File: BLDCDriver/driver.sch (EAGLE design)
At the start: 54 parts, among them Q1 NJM7800S, U1 QFN50P400X400X100-25NDRV8300D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, U2 AS5048A-HTSP-500, U4 SOP80P620X125-8N

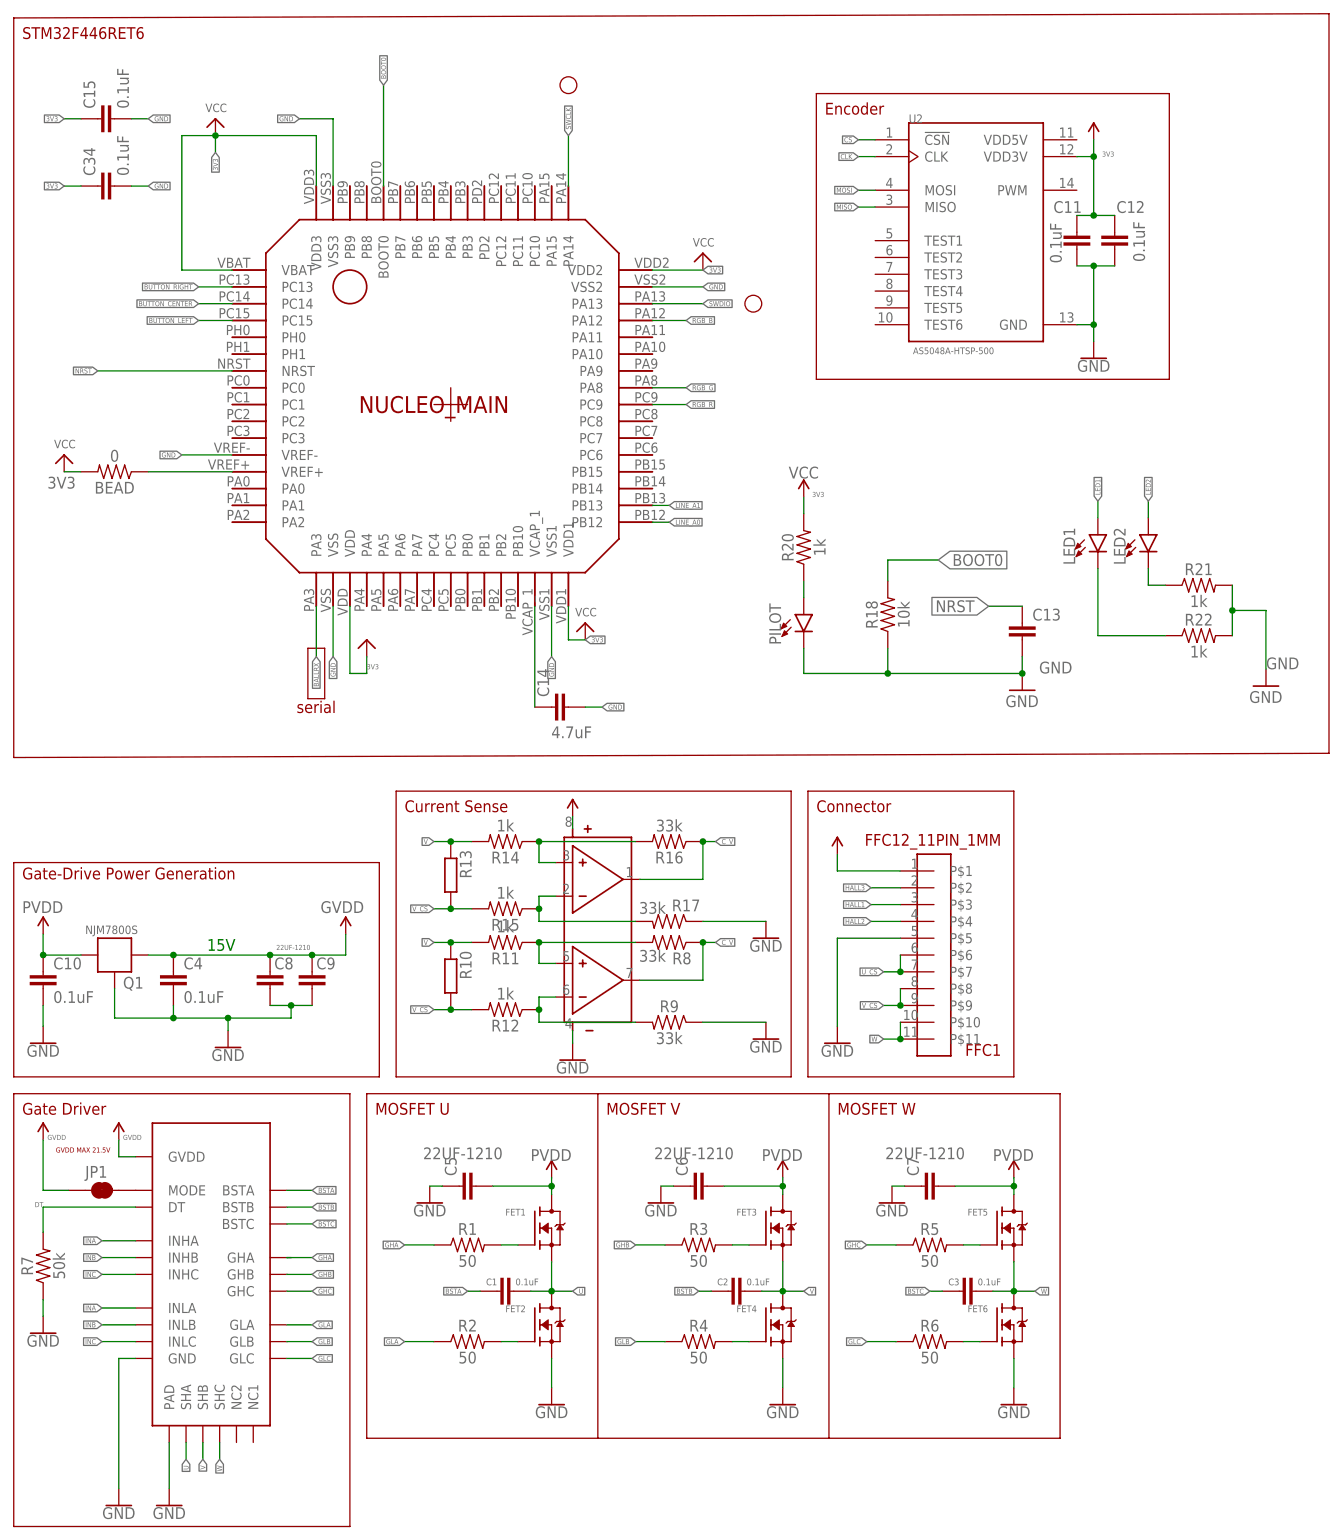
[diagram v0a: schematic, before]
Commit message: somefix
# ==== Emojis ====
# ✨ :sparkles: Add new feature
# ✅  :white_check_mark: Update existing feature (not bug)
# ⚠️  :warning: Fix bug/error
# 🔥  :fire: Remove files or features
# ✏️ :pencil2: Fix typos
# 📝  :memo: Update documentation
# ♻️  :recycle: Dependencies update
# 🐧  :penguin: Improved the Linux
# 🍎  :apple: Improved the macOS
# 🔖 :bookmark: Add new library
# 🎉  :tada: Initial commit

# ==== Format ====
# :emoji: Subject
#
# Commit body...

# ==== Messages ====
# 新規(ファイル)機能追加: Add
# 機能修正、既存機能追加（バグではない): Update
# リファクタリング: Clean
# ファイル名変更:
# 削除など: Remove
# バグ修正: Fix
# バージョンアップ: Upgrade
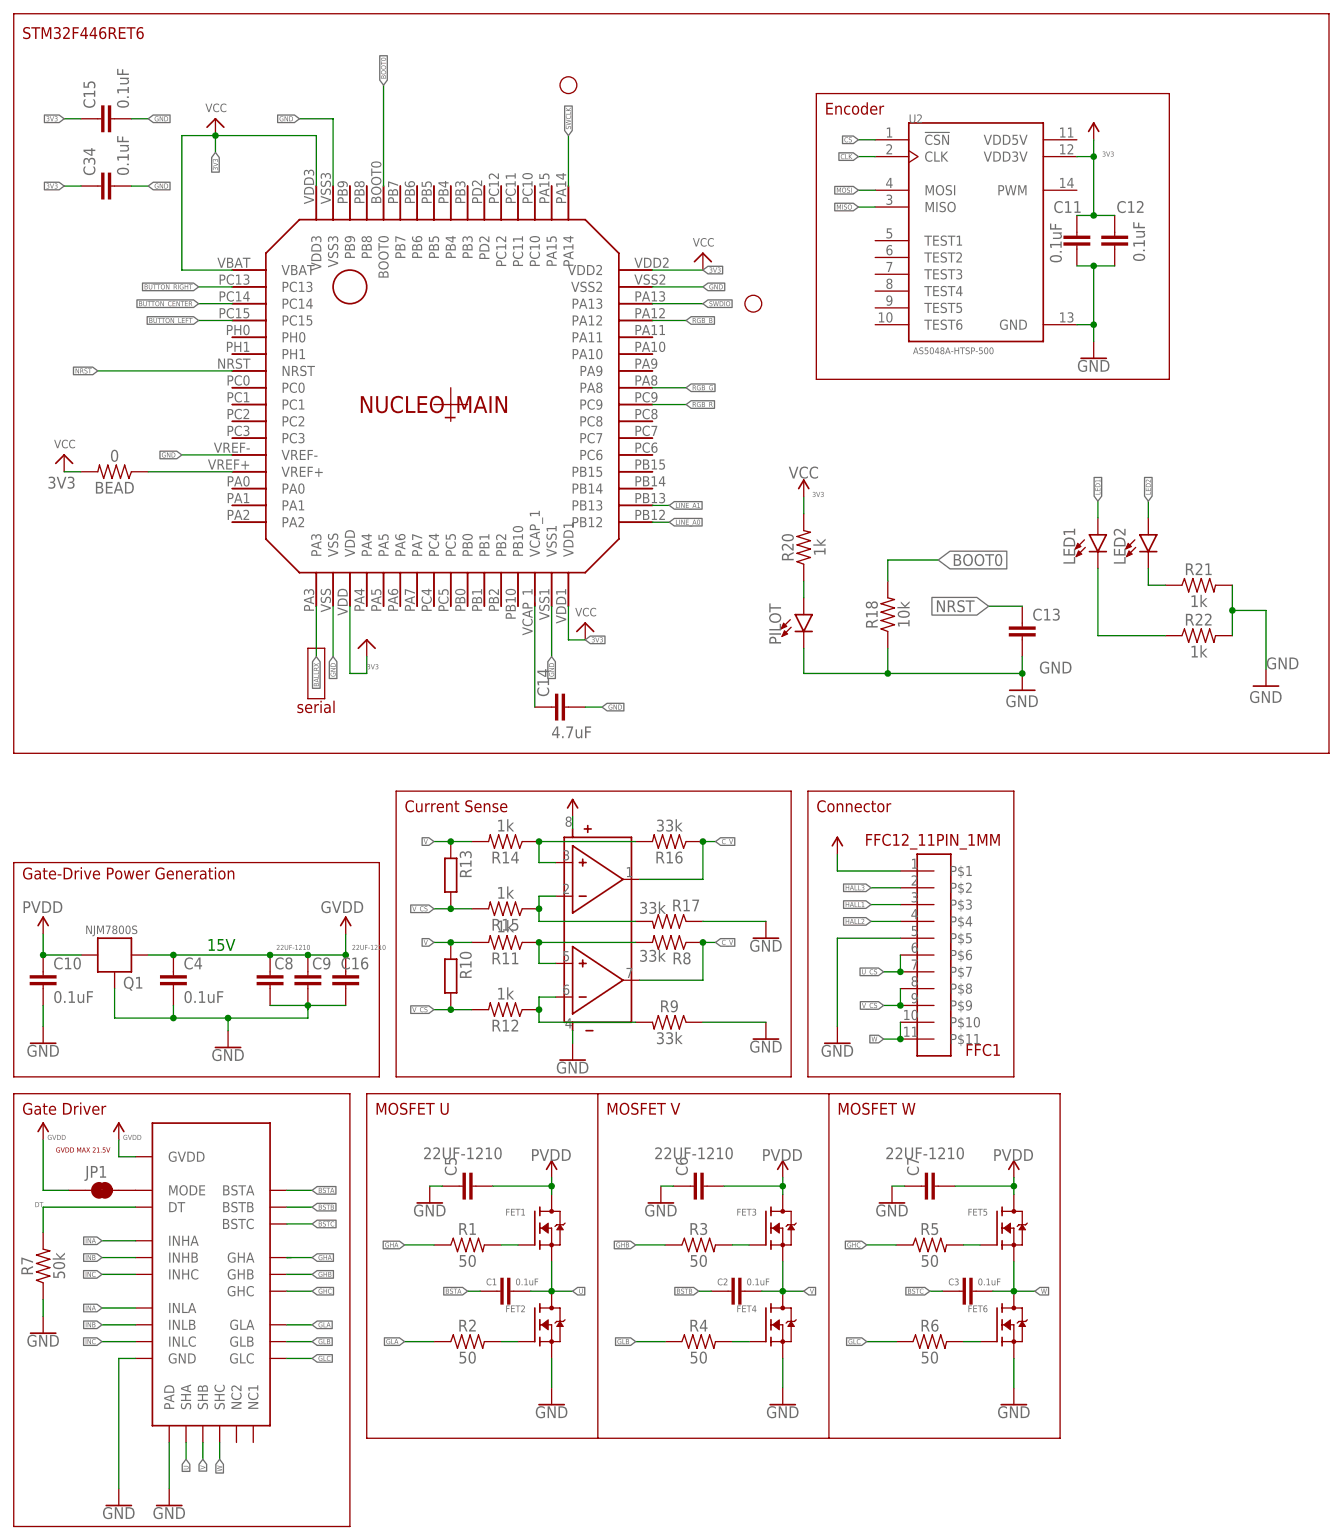
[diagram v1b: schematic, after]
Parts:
- added C16: 22UF-1210, SparkFun-Capacitors:22UF-1210-16V-20%
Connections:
- net GND: now also C16.1
- net GVDD: now also C16.2
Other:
- moved on the sheet: C9
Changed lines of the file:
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@@
 <part name="P+6" library="audio amplifier example" library_urn="urn:adsk.eagle:library:970892" deviceset="VCC" device=""/>
 <part name="GND18" library="supply" deviceset="GND" device=""/>
+<part name="C16" library="SparkFun-Capacitors" deviceset="22UF" device="-1210-16V-20%" value="22UF-1210"/>
 </parts>
 <sheets>
@@
 <circle x="83.82" y="217.805" radius="1.27" width="0.1524" layer="94"/>
 <circle x="111.76" y="184.785" radius="1.27" width="0.1524" layer="94"/>
-<wire x1="0" y1="227.965" x2="0" y2="116.205" width="0.1524" layer="94"/>
-<wire x1="0" y1="116.205" x2="198.755" y2="116.84" width="0.1524" layer="94"/>
+<wire x1="0" y1="228.6" x2="0" y2="116.84" width="0.1524" layer="94"/>
+<wire x1="0" y1="116.84" x2="198.755" y2="116.84" width="0.1524" layer="94"/>
 <wire x1="198.755" y1="116.84" x2="198.755" y2="228.6" width="0.1524" layer="94"/>
-<wire x1="198.755" y1="228.6" x2="0" y2="227.965" width="0.1524" layer="94"/>
+<wire x1="198.755" y1="228.6" x2="0" y2="228.6" width="0.1524" layer="94"/>
 <text x="1.27" y="224.79" size="1.778" layer="94">STM32F446RET6</text>
 </plain>
@@
 <attribute name="VALUE" x="44.831" y="87.884" size="0.762" layer="96" font="vector" rot="R180"/>
 </instance>
-<instance part="C9" gate="G$1" x="45.085" y="83.82" smashed="yes" rot="R180">
-<attribute name="NAME" x="48.641" y="85.979" size="1.778" layer="95" font="vector" rot="R180"/>
+<instance part="C9" gate="G$1" x="44.45" y="83.82" smashed="yes" rot="R180">
+<attribute name="NAME" x="48.006" y="85.979" size="1.778" layer="95" font="vector" rot="R180"/>
 </instance>
 <instance part="GND6" gate="1" x="32.385" y="72.39" smashed="yes">
@@
 <instance part="GND18" gate="1" x="189.23" y="127" smashed="yes">
 <attribute name="VALUE" x="186.69" y="124.46" size="1.778" layer="96"/>
+</instance>
+<instance part="C16" gate="G$1" x="50.165" y="83.82" smashed="yes" rot="R180">
+<attribute name="NAME" x="53.721" y="85.979" size="1.778" layer="95" font="vector" rot="R180"/>
+<attribute name="VALUE" x="56.261" y="87.884" size="0.762" layer="96" font="vector" rot="R180"/>
 </instance>
 </instances>
@@
 <wire x1="15.24" y1="81.28" x2="15.24" y2="76.835" width="0.1524" layer="91"/>
 <pinref part="C4" gate="G$1" pin="2"/>
-<pinref part="C8" gate="G$1" pin="1"/>
-<pinref part="C9" gate="G$1" pin="1"/>
-<wire x1="38.735" y1="78.74" x2="41.91" y2="78.74" width="0.1524" layer="91"/>
-<wire x1="41.91" y1="78.74" x2="45.085" y2="78.74" width="0.1524" layer="91"/>
-<wire x1="41.91" y1="78.74" x2="41.91" y2="76.835" width="0.1524" layer="91"/>
-<junction x="41.91" y="78.74"/>
 <wire x1="24.13" y1="76.835" x2="24.13" y2="78.74" width="0.1524" layer="91"/>
 <wire x1="24.13" y1="76.835" x2="15.24" y2="76.835" width="0.1524" layer="91"/>
@@
 <pinref part="GND6" gate="1" pin="GND"/>
 <wire x1="24.13" y1="76.835" x2="32.385" y2="76.835" width="0.1524" layer="91"/>
-<wire x1="32.385" y1="76.835" x2="41.91" y2="76.835" width="0.1524" layer="91"/>
+<wire x1="32.385" y1="76.835" x2="44.45" y2="76.835" width="0.1524" layer="91"/>
 <wire x1="32.385" y1="74.93" x2="32.385" y2="76.835" width="0.1524" layer="91"/>
 <junction x="32.385" y="76.835"/>
+<pinref part="C9" gate="G$1" pin="1"/>
+<pinref part="C16" gate="G$1" pin="1"/>
+<wire x1="50.165" y1="78.74" x2="44.45" y2="78.74" width="0.1524" layer="91"/>
+<junction x="44.45" y="78.74"/>
+<pinref part="C8" gate="G$1" pin="1"/>
+<wire x1="38.735" y1="78.74" x2="44.45" y2="78.74" width="0.1524" layer="91"/>
+<wire x1="44.45" y1="78.105" x2="44.45" y2="78.74" width="0.1524" layer="91"/>
+<wire x1="44.45" y1="78.74" x2="44.45" y2="76.835" width="0.1524" layer="91"/>
 </segment>
 <segment>
@@
 <pinref part="C8" gate="G$1" pin="2"/>
 <junction x="38.735" y="86.36"/>
-<wire x1="38.735" y1="86.36" x2="45.085" y2="86.36" width="0.1524" layer="91"/>
+<wire x1="38.735" y1="86.36" x2="44.45" y2="86.36" width="0.1524" layer="91"/>
 <pinref part="C9" gate="G$1" pin="2"/>
-<junction x="45.085" y="86.36"/>
-<wire x1="45.085" y1="86.36" x2="50.165" y2="86.36" width="0.1524" layer="91"/>
+<junction x="44.45" y="86.36"/>
+<wire x1="44.45" y1="86.36" x2="50.165" y2="86.36" width="0.1524" layer="91"/>
 <wire x1="50.165" y1="86.36" x2="50.165" y2="89.535" width="0.1524" layer="91"/>
+<pinref part="C16" gate="G$1" pin="2"/>
+<junction x="50.165" y="86.36"/>
 </segment>
 </net>
